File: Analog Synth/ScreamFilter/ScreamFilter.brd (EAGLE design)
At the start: 46.4 x 63.5 mm, 37 parts, among them IC1 TL084P, IC2 TL082P, Q1 J310, Q2 J310, Q3 J310, Q4 J310

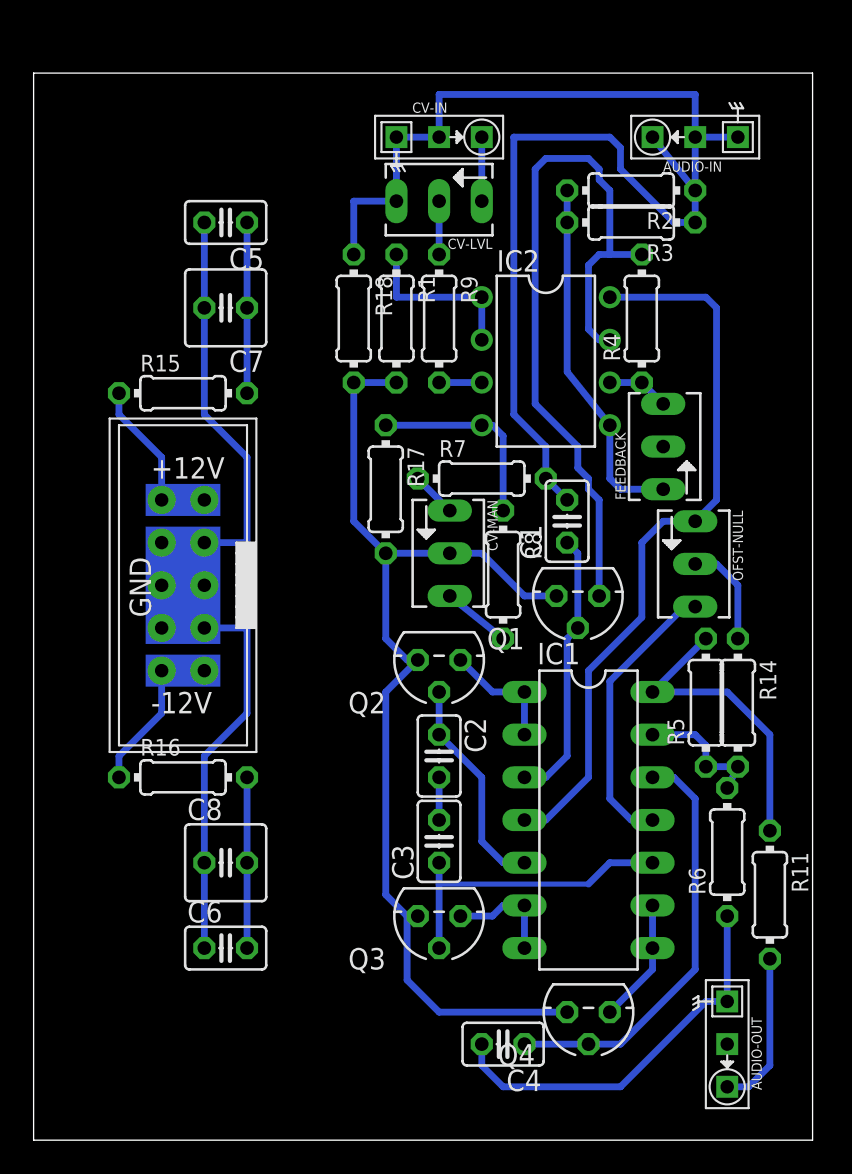
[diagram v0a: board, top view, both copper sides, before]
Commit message: working on ScreamFilter DIY layout
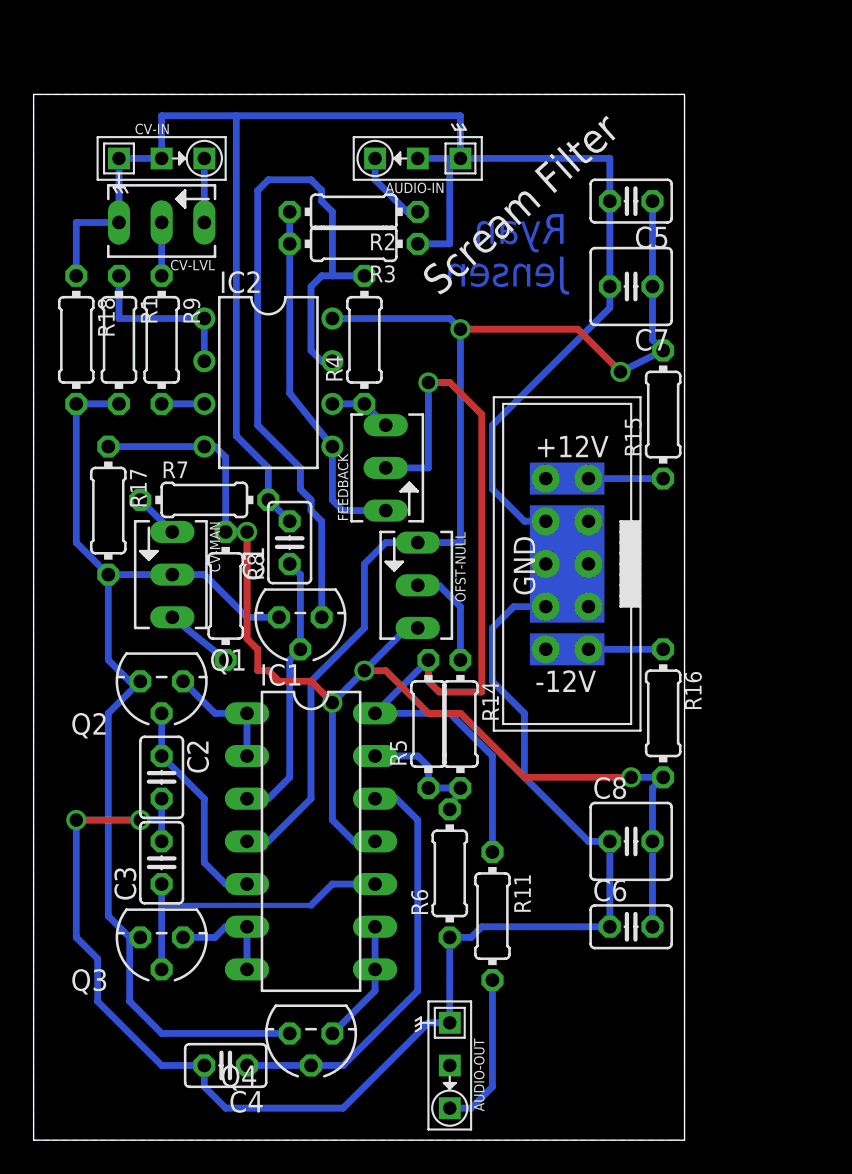
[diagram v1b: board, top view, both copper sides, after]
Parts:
- moved R16 28.8 mm to (37.5, 25.4), turned to 270 degrees
- moved R15 28.6 mm to (37.5, 43.2), turned to 90 degrees
- moved C5 24.2 mm to (35.6, 55.9)
- moved C6 24.2 mm to (35.6, 12.7)
- moved C7 24.2 mm to (35.6, 50.8)
- moved C8 24.2 mm to (35.6, 17.8)
- moved U$1 22.9 mm to (31.8, 34.3)
- moved FEEDBACK 16.6 mm to (21.0, 40.0)
- moved C4 16.6 mm to (11.4, 4.45)
- moved IC1 16.6 mm to (16.5, 17.8)
- moved Q4 16.6 mm to (16.5, 6.35)
- moved R18 16.6 mm to (2.54, 47.6)
- moved R2 16.6 mm to (19.1, 55.2)
- moved R3 16.6 mm to (19.1, 53.3)
- moved R4 16.6 mm to (19.7, 47.6)
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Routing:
- net GND: track 148.0 -> 204.0 mm, vias 0 -> 2
- net -12V: track 38.8 -> 73.3 mm, vias 0 -> 4
- net N$10: track 18.2 -> 51.0 mm, vias 0 -> 1
- net +12V: track 53.8 -> 69.5 mm, vias 0 -> 2
- net N$1: track 4.07 -> 4.60 mm
- added copper zone on layer 16, net GND
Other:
- board size 46.4 x 63.5 mm -> 38.7 x 62.2 mm
- board text added: "Jensen"
- board text added: "Ryan"
- board text added: "Scream Filter"
